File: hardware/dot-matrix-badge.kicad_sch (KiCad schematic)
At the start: 5 parts, among them J1 AVR-ISP-6, SW1 SW_SPST, U1 ATtiny13A-SS

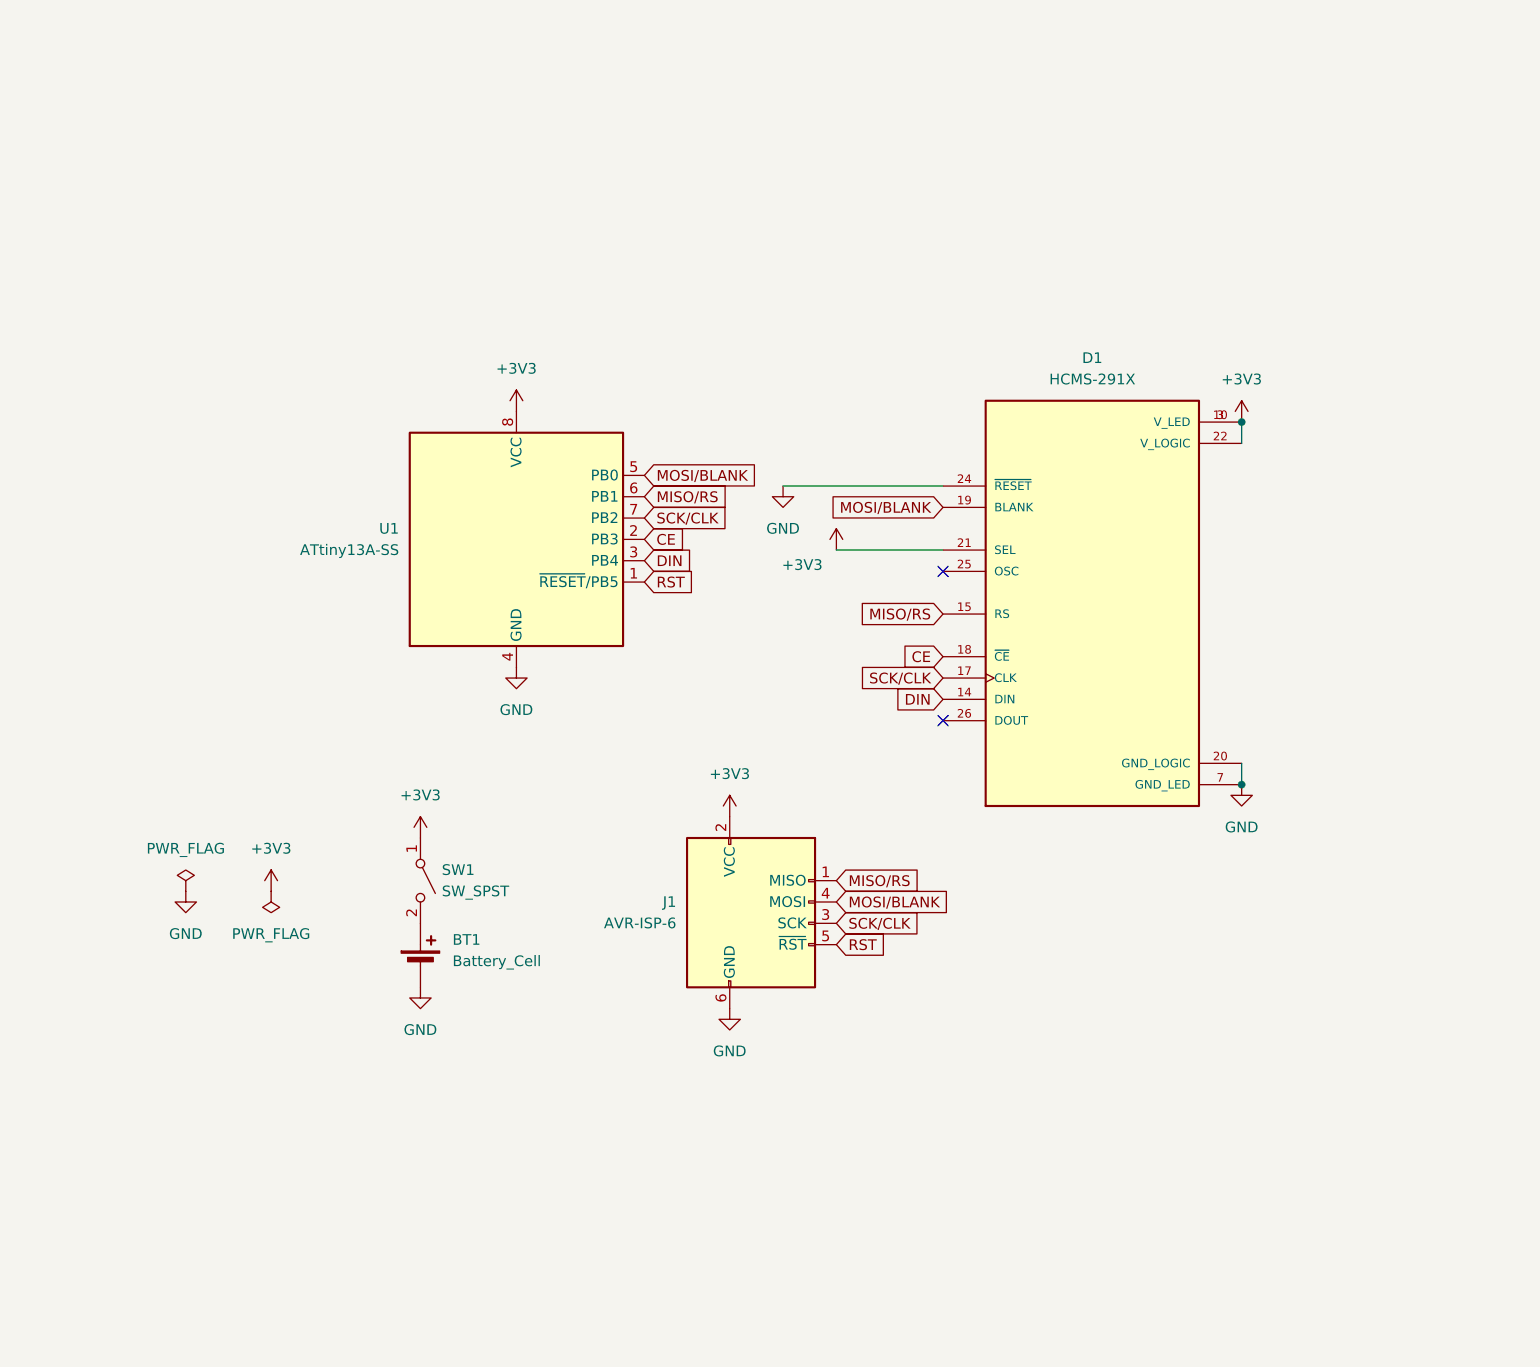
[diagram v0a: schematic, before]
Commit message: cpp firmware, hardware progress
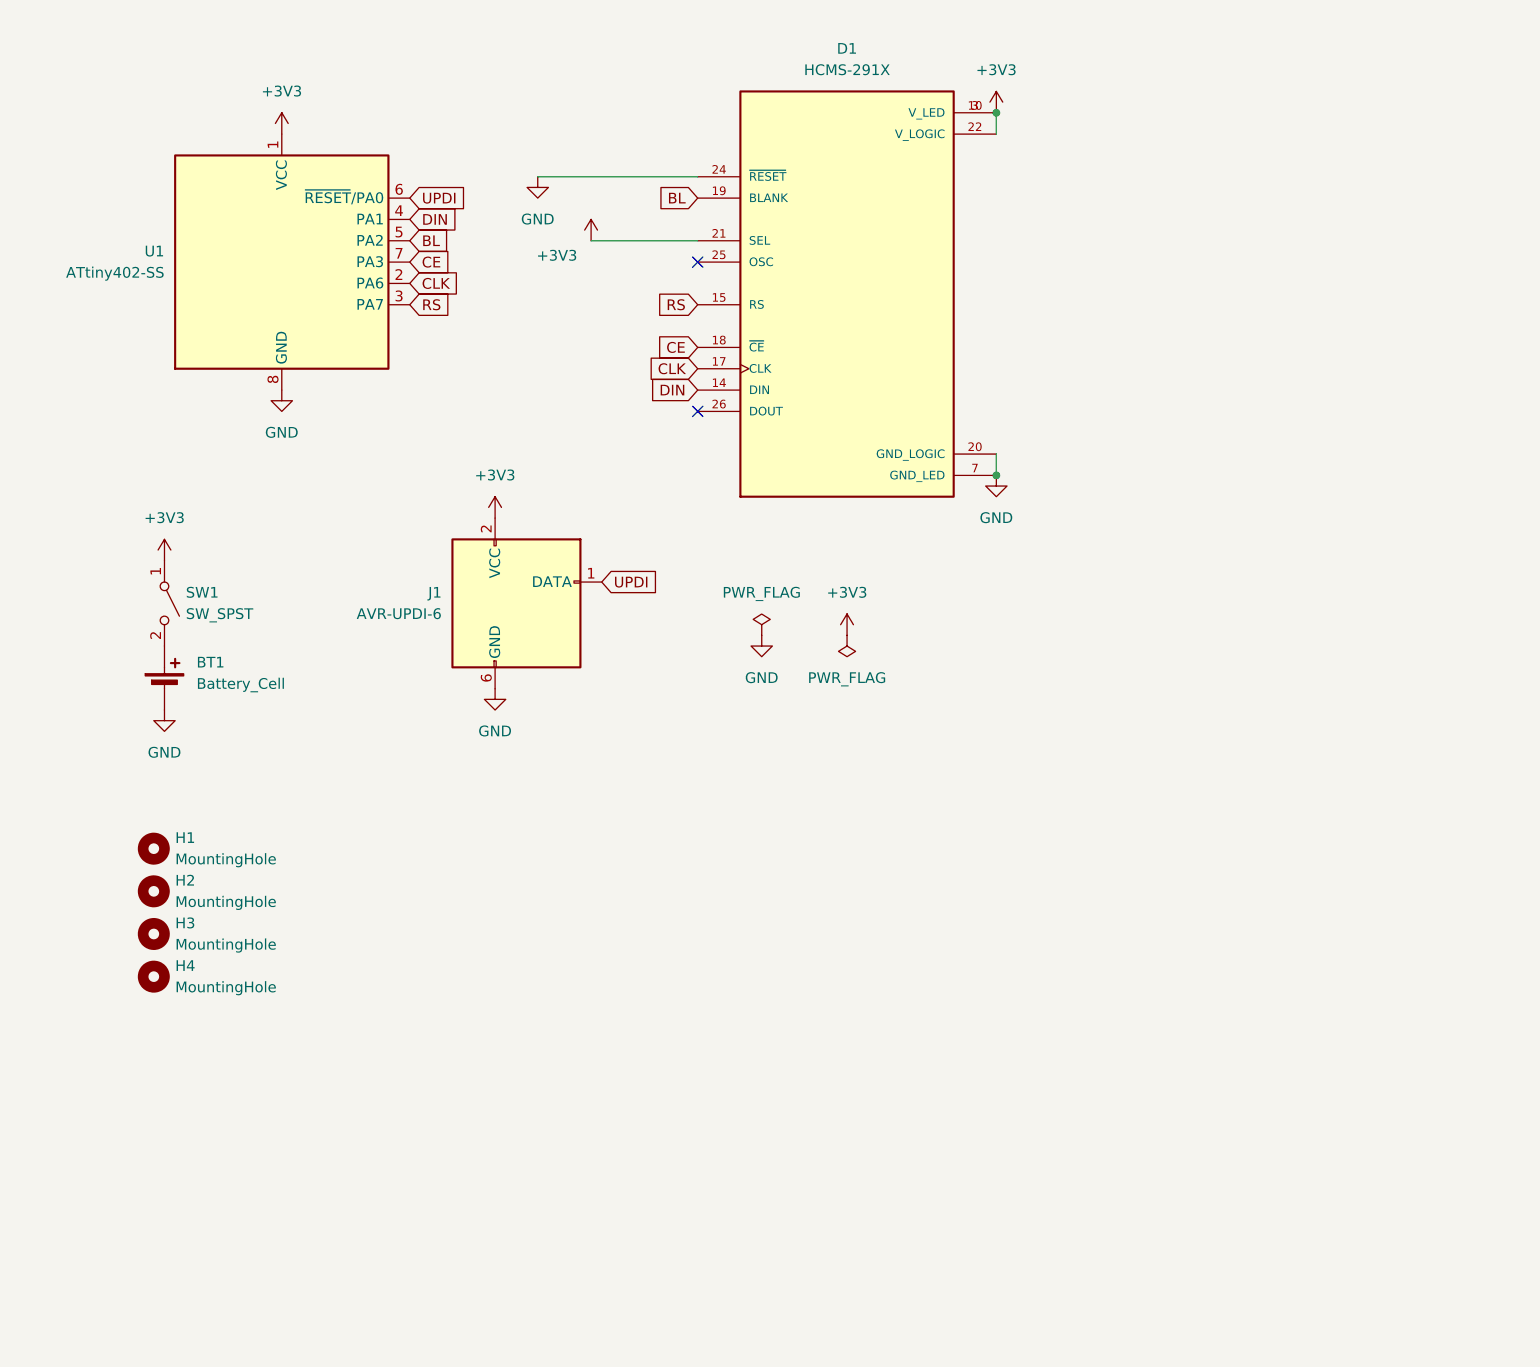
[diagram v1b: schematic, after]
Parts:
- removed J1: AVR-ISP-6, Connector_PinSocket_2.54mm:PinSocket_2x03_P2.54mm_Vertical, symbol Connector:AVR-ISP-6
- removed U1: ATtiny13A-SS, Package_SO:SOIC-8_3.9x4.9mm_P1.27mm, symbol MCU_Microchip_ATtiny:ATtiny13A-SS
- added H1, H2, H3, H4: MountingHole, DotMatrixBadge:MountingHole_Custom, symbol Mechanical:MountingHole
- added J1: AVR-UPDI-6, DotMatrixBadge:UPDI_Pads, symbol Connector:AVR-UPDI-6
- added U1: ATtiny402-SS, Package_SO:SOIC-8_3.9x4.9mm_P1.27mm, symbol MCU_Microchip_ATtiny:ATtiny402-SS
- BT1: footprint Battery:BatteryHolder_Multicomp_BC-2001_1x2032 -> Battery:BatteryHolder_Keystone_3034_1x20mm
- D1: footprint HCMS-291x:HCMS-291X -> DotMatrixBadge:HCMS-291X; symbol HCMS-291X:HCMS-291X -> DotMatrixBadge:HCMS-291X
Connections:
- net +3V3: now also J1.2 (VCC), U1.1 (VCC)
- net CE: now also U1.7 (PA3)
- net DIN: now also U1.4 (PA1)
- net GND: now also J1.6 (GND), U1.8 (GND)
- net MISO/RS renamed RS
- net RS: now also U1.3 (PA7)
- net MOSI/BLANK renamed BL
- net BL: now also U1.5 (PA2)
- net SCK/CLK renamed CLK
- net CLK: now also U1.2 (PA6)
- new net UPDI: J1.1 (DATA), U1.6 (~{RESET}/PA0)
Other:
- moved on the sheet: BT1, D1, SW1

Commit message: almost done with layout
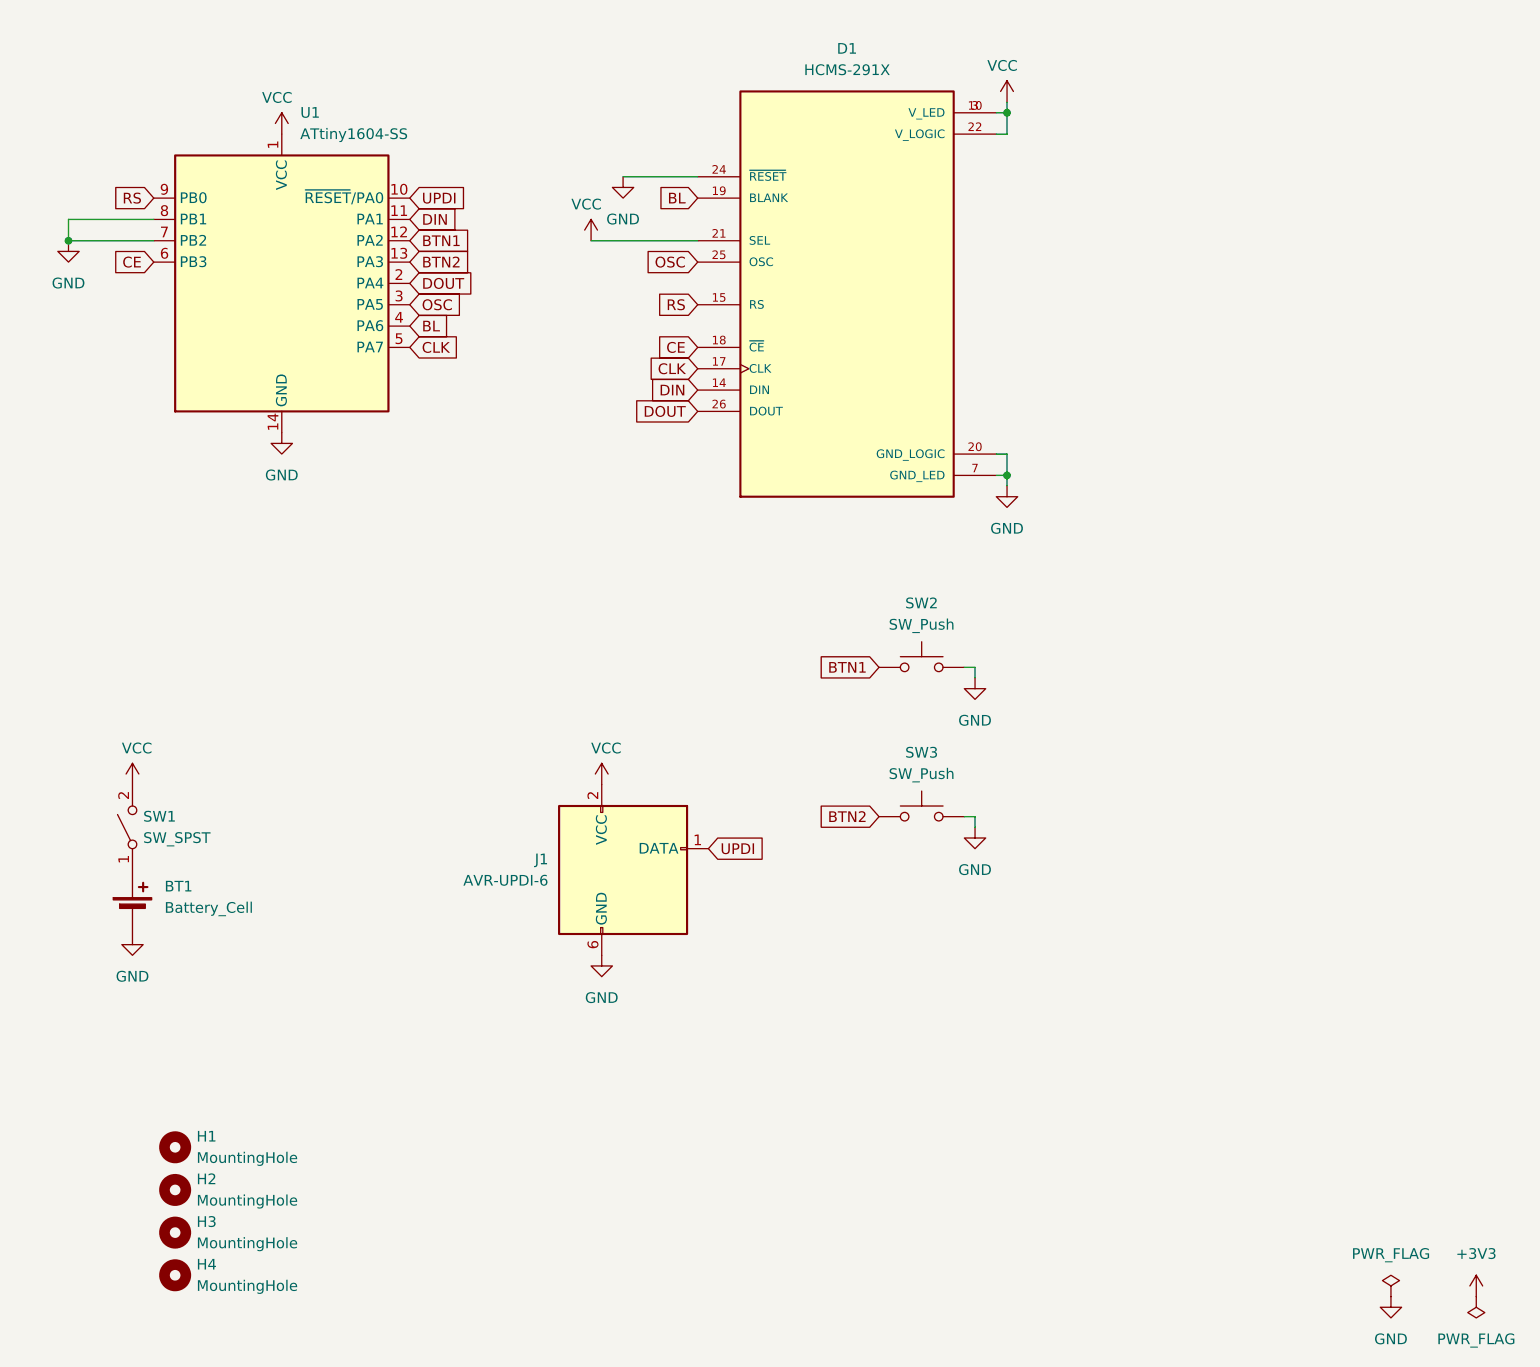
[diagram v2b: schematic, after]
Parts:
- removed U1: ATtiny402-SS, Package_SO:SOIC-8_3.9x4.9mm_P1.27mm, symbol MCU_Microchip_ATtiny:ATtiny402-SS
- added SW2, SW3: SW_Push, DotMatrixBadge:SW_SPST_PTS526_JLeads, symbol Switch:SW_Push
- added U1: ATtiny1604-SS, Package_SO:SOIC-14_3.9x8.7mm_P1.27mm, symbol MCU_Microchip_ATtiny:ATtiny1604-SS
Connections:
- net +3V3: no longer D1.10 (V_LED), D1.21 (SEL), D1.22 (V_LOGIC), D1.3 (V_LED), J1.2 (VCC), SW1.1 (A)
- net BL: now also U1.4 (PA6)
- net CE: now also U1.6 (PB3)
- net CLK: now also U1.5 (PA7)
- net DIN: now also U1.11 (PA1)
- net GND: now also SW2.2, SW3.2, U1.14 (GND), U1.7 (PB2), U1.8 (PB1)
- net RS: now also U1.9 (PB0)
- net UPDI: now also U1.10 (~{RESET}/PA0)
- net at BT1.1 (+): now also SW1.1 (A); no longer SW1.2 (B)
- net OSC: now reaches D1.25 (OSC)
- net OSC: now also U1.3 (PA5)
- net DOUT: now reaches D1.26 (DOUT)
- net DOUT: now also U1.2 (PA4)
- new net BTN1: SW2.1, U1.12 (PA2)
- new net BTN2: SW3.1, U1.13 (PA3)
- new net VCC: D1.10 (V_LED), D1.21 (SEL), D1.22 (V_LOGIC), D1.3 (V_LED), J1.2 (VCC), SW1.2 (B), U1.1 (VCC)
- no-connect marks 2 -> 0
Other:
- moved on the sheet: BT1, H1, H2, H3, H4, J1, SW1

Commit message: pcb payout almost complete
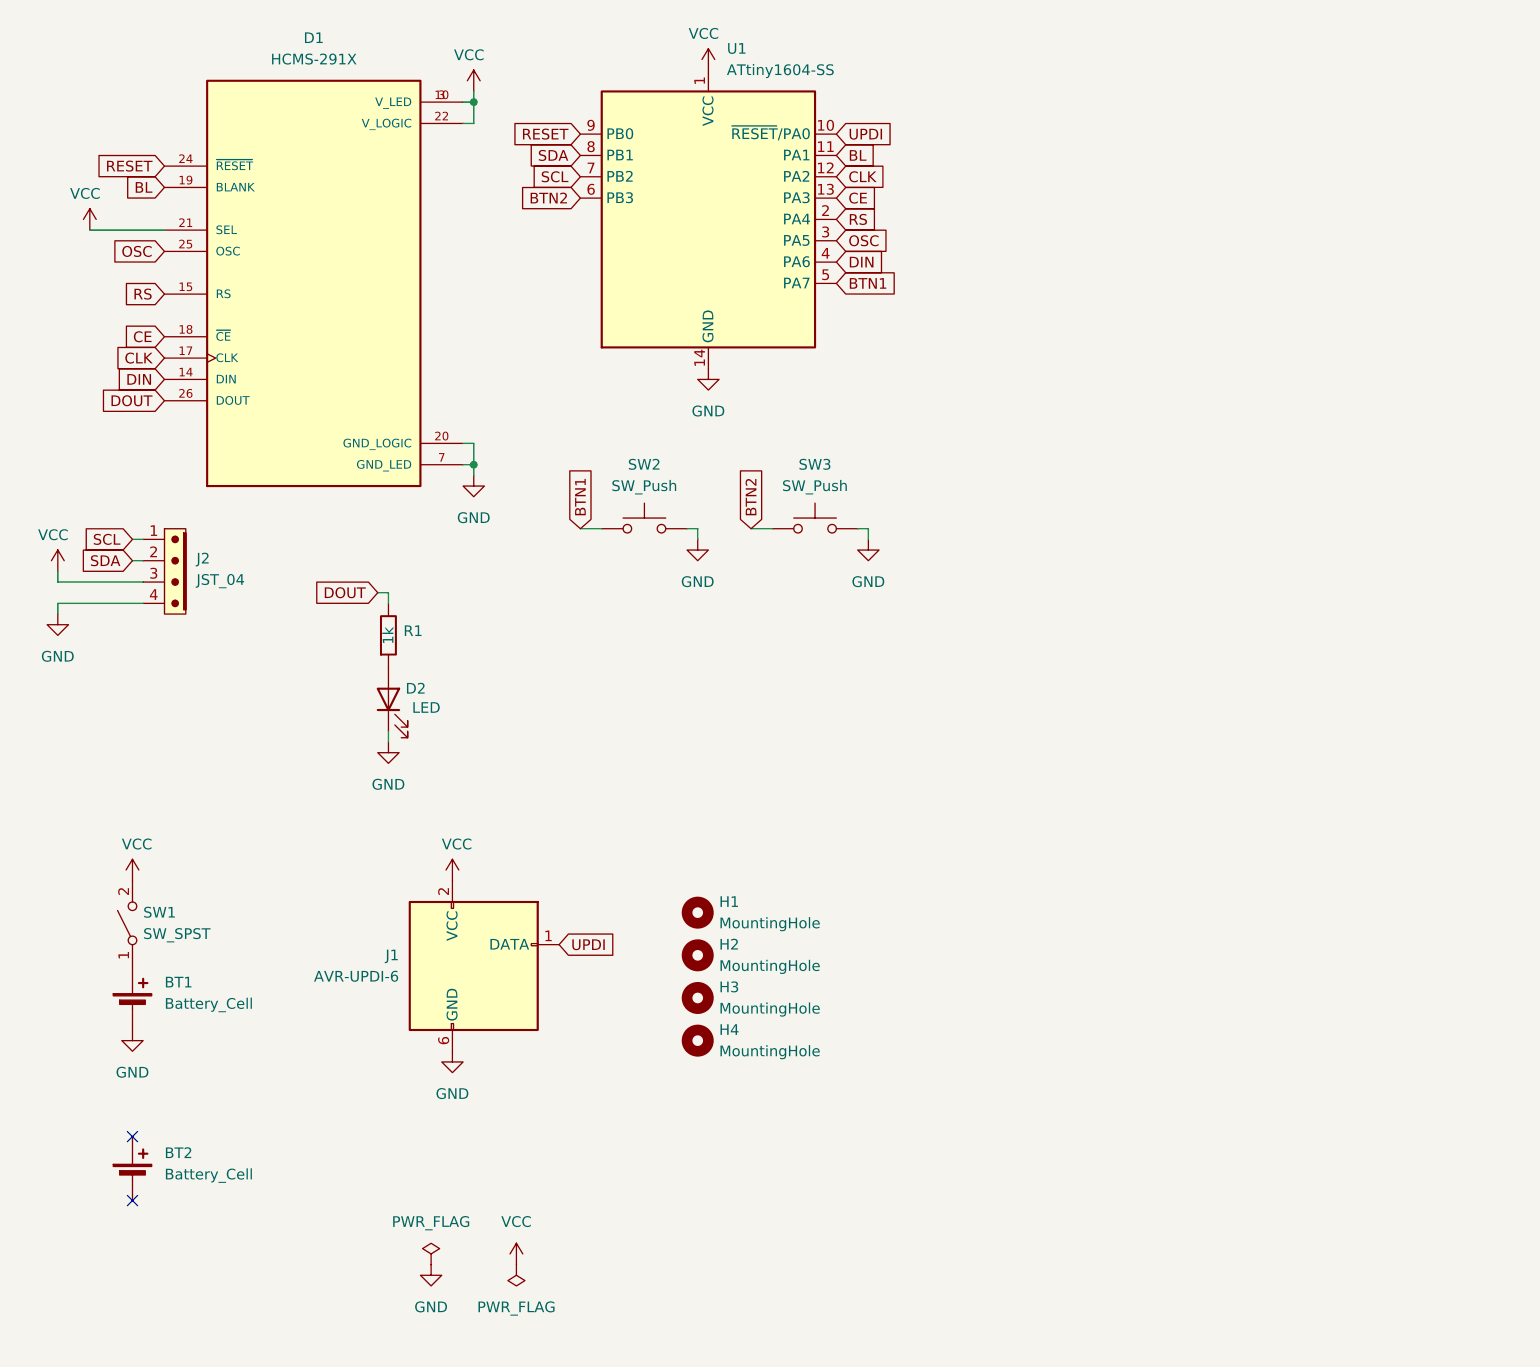
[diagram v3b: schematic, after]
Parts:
- added BT2: Battery_Cell, DotMatrixBadge:SpareBatteryHolder_Keystone_3034_1x20mm, symbol Device:Battery_Cell
- added D2: LED, LED_SMD:LED_0603_1608Metric, symbol Device:LED
- added J2: JST_04, Connector_JST:JST_SH_BM04B-SRSS-TB_1x04-1MP_P1.00mm_Vertical, symbol PCM_SL_Connectors:JST_04
- added R1: 1k, Resistor_SMD:R_0402_1005Metric, symbol PCM_SL_Resistors:Resistor
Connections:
- net BL: now also U1.11 (PA1); no longer U1.4 (PA6)
- net BTN1: now also U1.5 (PA7); no longer U1.12 (PA2)
- net BTN2: now also U1.6 (PB3); no longer U1.13 (PA3)
- net CE: now also U1.13 (PA3); no longer U1.6 (PB3)
- net CLK: now also U1.12 (PA2); no longer U1.5 (PA7)
- net DIN: now also U1.4 (PA6); no longer U1.11 (PA1)
- net DOUT: now also R1.2; no longer U1.2 (PA4)
- net GND: now also D2.1 (K), J2.4; no longer D1.24 (~{RESET}), U1.7 (PB2), U1.8 (PB1)
- net RS: now also U1.2 (PA4); no longer U1.9 (PB0)
- net VCC: now also J2.3
- new net: D2.2 (A), R1.1
- new net RESET: D1.24 (~{RESET}), U1.9 (PB0)
- new net SCL: J2.1, U1.7 (PB2)
- new net SDA: J2.2, U1.8 (PB1)
- no-connect marks 0 -> 2
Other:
- moved on the sheet: BT1, D1, H1, H2, H3, H4, J1, SW1, SW2, SW3, U1
